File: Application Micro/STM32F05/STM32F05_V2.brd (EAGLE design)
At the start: 100 x 80 mm, 40 parts, among them T1 FDN340P, T2 AP1117_LIN_REG

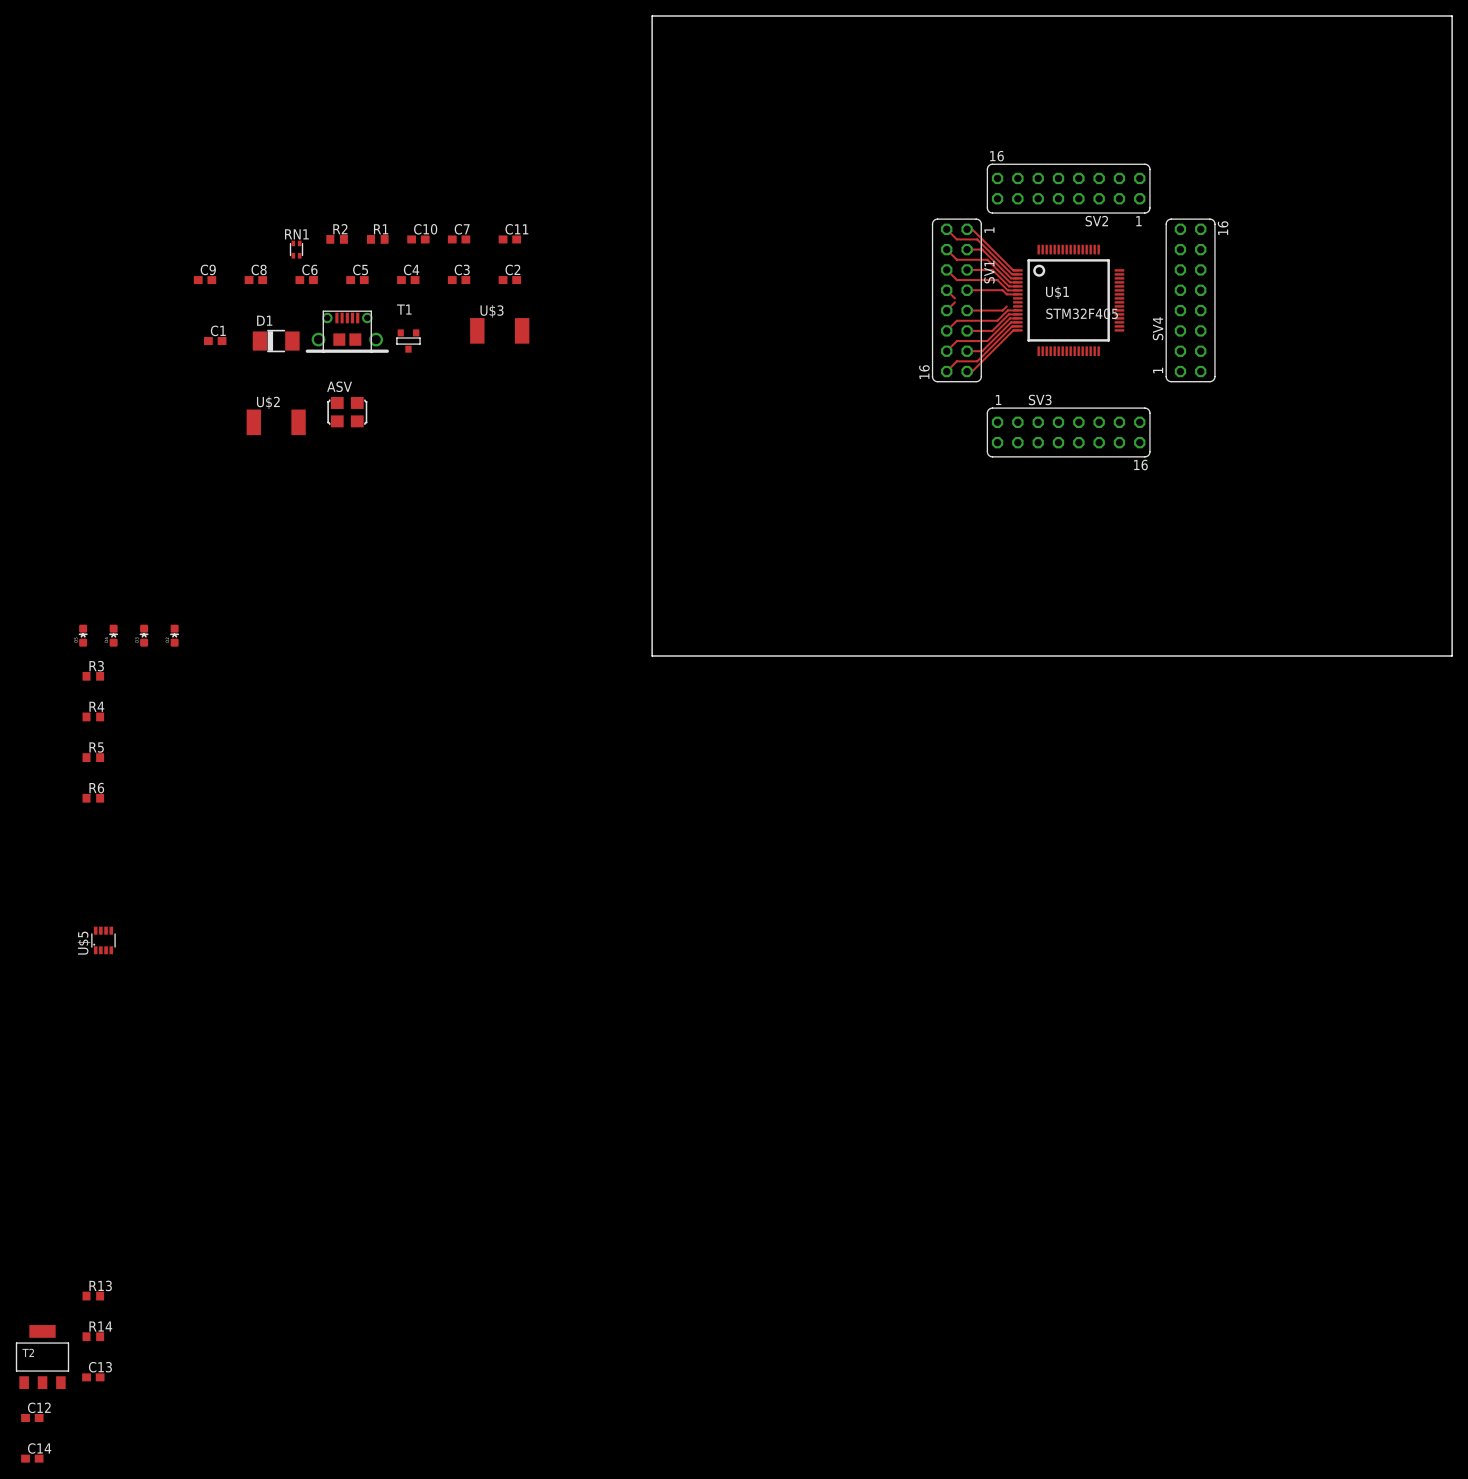
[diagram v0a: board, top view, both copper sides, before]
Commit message: Started Routing
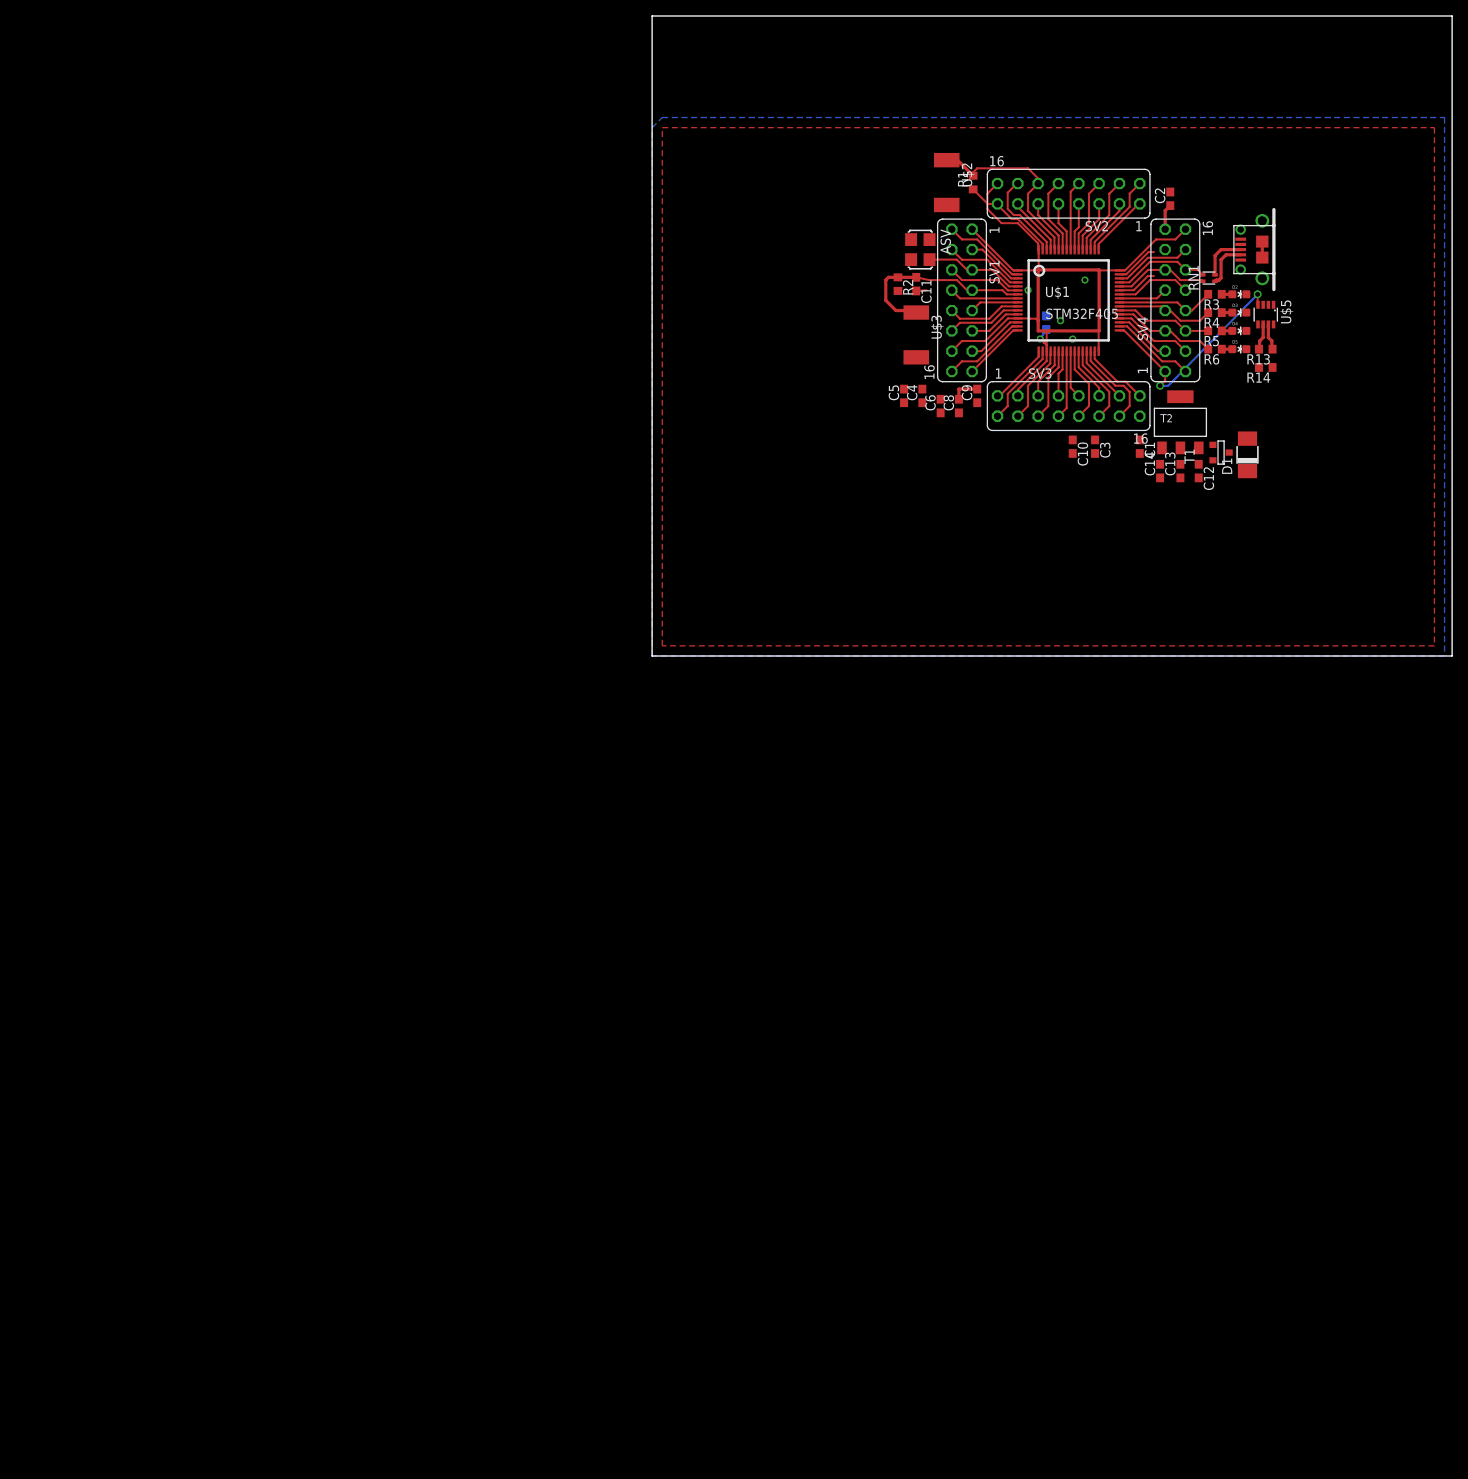
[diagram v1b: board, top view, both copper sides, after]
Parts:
- R3, R4, R6: value 10K -> 82
- R5: value 10K -> 10
- moved R14 190.2 mm to (76.7, 36.1), turned to 180 degrees
- moved R13 188.4 mm to (76.7, 38.4), turned to 180 degrees
- moved C12 187.8 mm to (68.3, 23.1), turned to 270 degrees
- moved C14 187.4 mm to (63.5, 23.1), turned to 90 degrees
- moved T2 184.1 mm to (66.0, 29.2)
- moved C13 176.9 mm to (66.0, 23.1), turned to 90 degrees
- moved U$5 165.0 mm to (76.7, 42.7), turned to 180 degrees
- moved R6 151.0 mm to (70.4, 38.4), turned to 180 degrees
- moved R5 150.0 mm to (70.4, 40.6), turned to 180 degrees
- moved R4 149.0 mm to (70.4, 42.9), turned to 180 degrees
- moved D5 148.9 mm to (73.4, 38.4), turned to 270 degrees
- moved R3 148.1 mm to (70.4, 45.2), turned to 180 degrees
- moved D4 145.8 mm to (73.4, 40.6), turned to 270 degrees
- moved D3 142.7 mm to (73.4, 42.9), turned to 270 degrees
- moved D2 139.8 mm to (73.4, 45.2), turned to 270 degrees
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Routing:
- net +3V3: track 19.1 -> 96.5 mm, vias 0 -> 1
- net GND: track 7.20 -> 46.7 mm, vias 0 -> 4
- net CAN2_RX: track 0.00 -> 28.2 mm, vias 0 -> 2
- net BOOT0: track 0.00 -> 24.5 mm
- net NRST: track 6.57 -> 24.4 mm
- net DBUG_LED4: track 0.00 -> 12.9 mm
- net DBUG_LED1: track 0.00 -> 12.4 mm
- net DBUG_LED2: track 0.00 -> 12.3 mm
- net DBUG_LED3: track 0.00 -> 12.1 mm
- net USBD+: track 0.00 -> 12.1 mm
- net USBD-: track 0.00 -> 11.8 mm
- net PIN62: track 0.00 -> 11.3 mm
- net PIN30: track 0.00 -> 11.3 mm
- net PIN50: track 0.00 -> 10.6 mm
- net CAN2_TX: track 0.00 -> 10.6 mm
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- added copper zone on layer 1, net GND
- added copper zone on layer 16, net GND
